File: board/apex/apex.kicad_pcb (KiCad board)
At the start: 4 copper layers, 65.4 x 30.5 mm, 11 parts, among them J1 USB_C_Receptacle_PowerOnly_6P

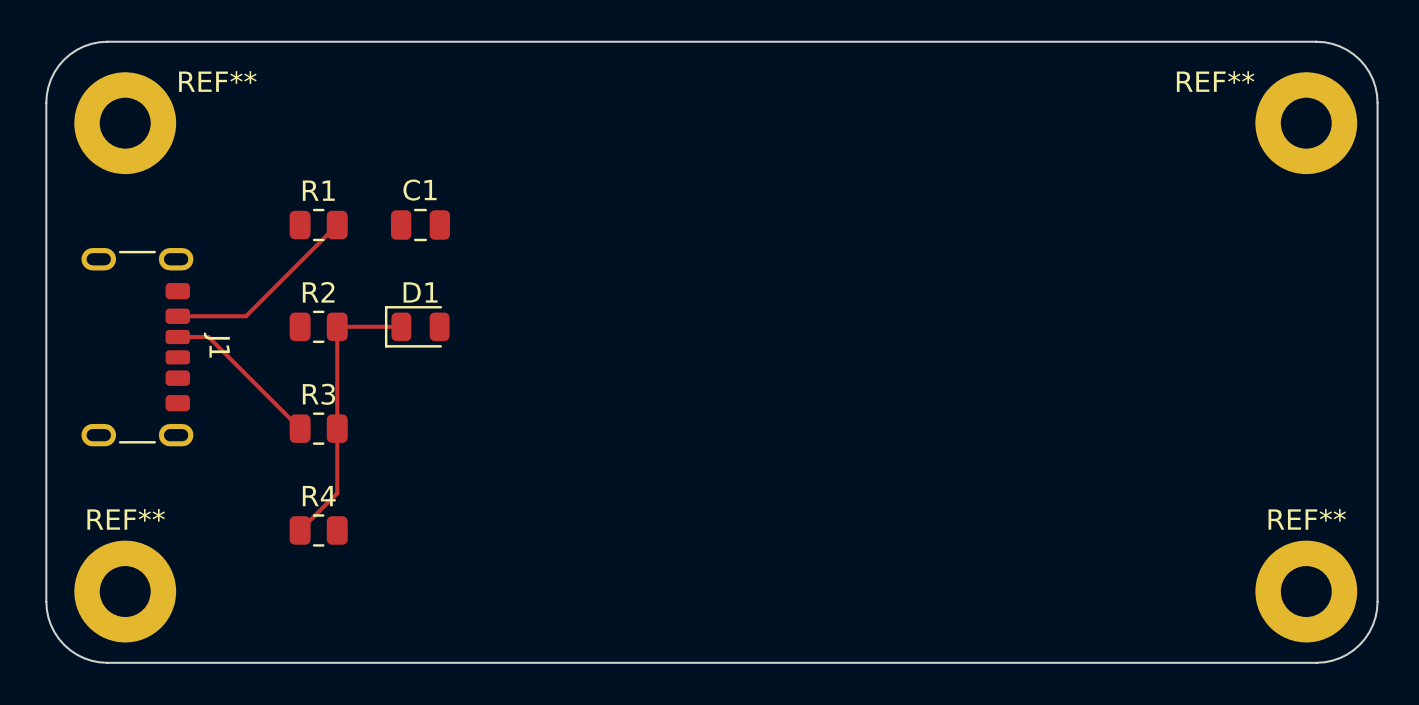
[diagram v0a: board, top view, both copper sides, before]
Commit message: organized modules
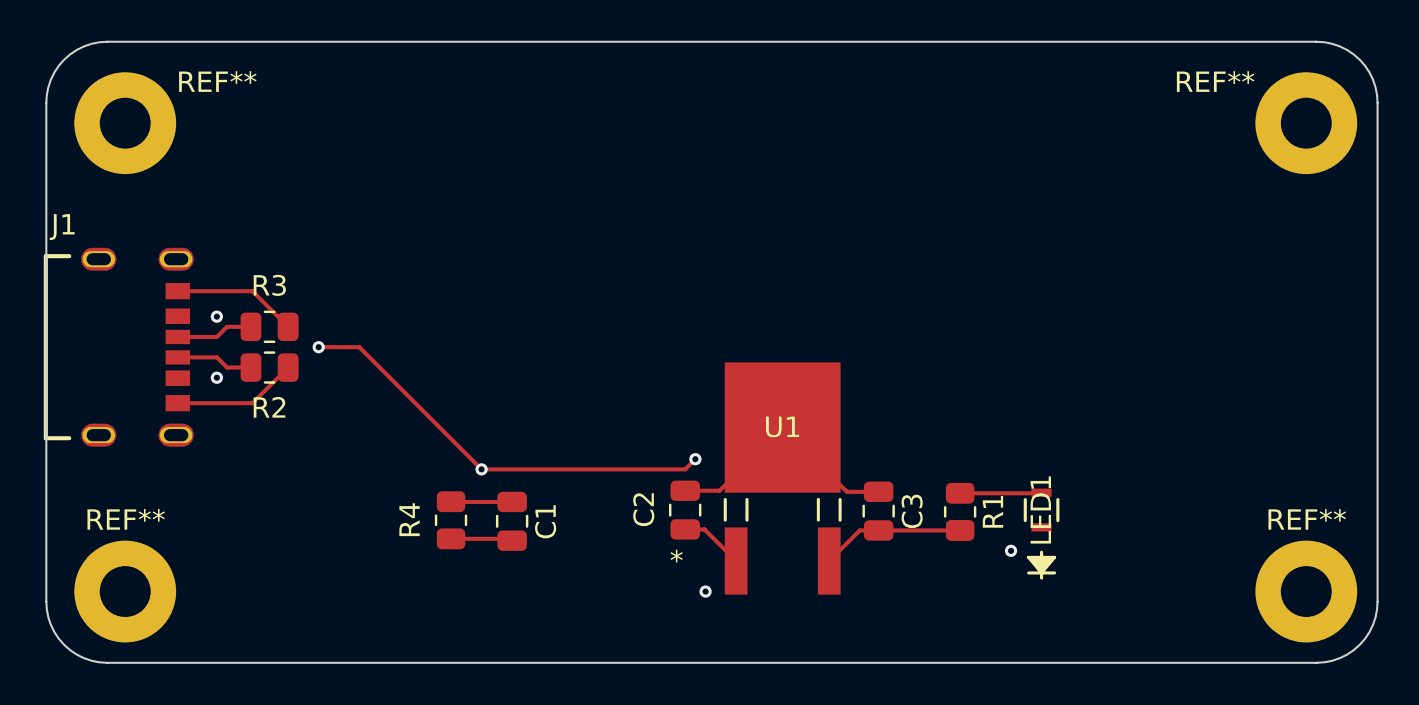
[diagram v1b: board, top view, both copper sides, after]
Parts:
- removed D1: LED, LED_SMD:LED_0805_2012Metric
- added C2: 10 uF, Capacitor_SMD:C_0805_2012Metric, F.Cu at (48.0, 54.0)
- added C3: 10 uF, Capacitor_SMD:C_0805_2012Metric, F.Cu at (57.5, 54.0)
- added LED1: 150080BS75000, LEDBS75000_WRE:LED_BS75000_WRE, F.Cu at (65.5, 54.0)
- added U1: AP7363-33D-13, AP7363_33D_13:TO252-3L_DIO, F.Cu at (52.8, 49.9)
- C1: value 0.1uF -> 0.1 uF
- J1: value USB_C_Receptacle_PowerOnly_6P -> USB4125-GF-A_REVA2; footprint Connector_USB:USB_C_Receptacle_GCT_USB4125-xx-x-0190_6P_TopMnt_Horizontal -> USB4125_GF_A:GCT_USB4125-GF-A_REVA2
- R1: value R -> 3.3
- moved R1 34.5 mm to (61.5, 54.1), turned to -90 degrees
- moved C1 15.2 mm to (39.5, 54.5), turned to -90 degrees
- moved R4 6.52 mm to (36.5, 54.5), turned to -90 degrees
- moved R3 5.55 mm to (27.6, 45.0)
- moved R2 3.13 mm to (27.6, 47.0)
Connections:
- R1 pad 2: VBUS -> +3V3
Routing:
- net (no net): track 0.00 -> 21.2 mm, vias 0 -> 7
- net GND: track 13.9 -> 27.4 mm
- net +3V3: track 0.00 -> 7.05 mm
- net VBUS: track 9.69 -> 3.14 mm
- net Net-(J1-CC1): track 7.87 -> 3.80 mm
- net Net-(LED1-Pad2): track 0.00 -> 4.01 mm
- net Net-(J1-CC2): track 0.00 -> 3.80 mm
- net GNDPWR: track 0.00 -> 3.04 mm
